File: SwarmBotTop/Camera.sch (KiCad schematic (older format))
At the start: 3 parts, among them J6 Conn_01x24_Female

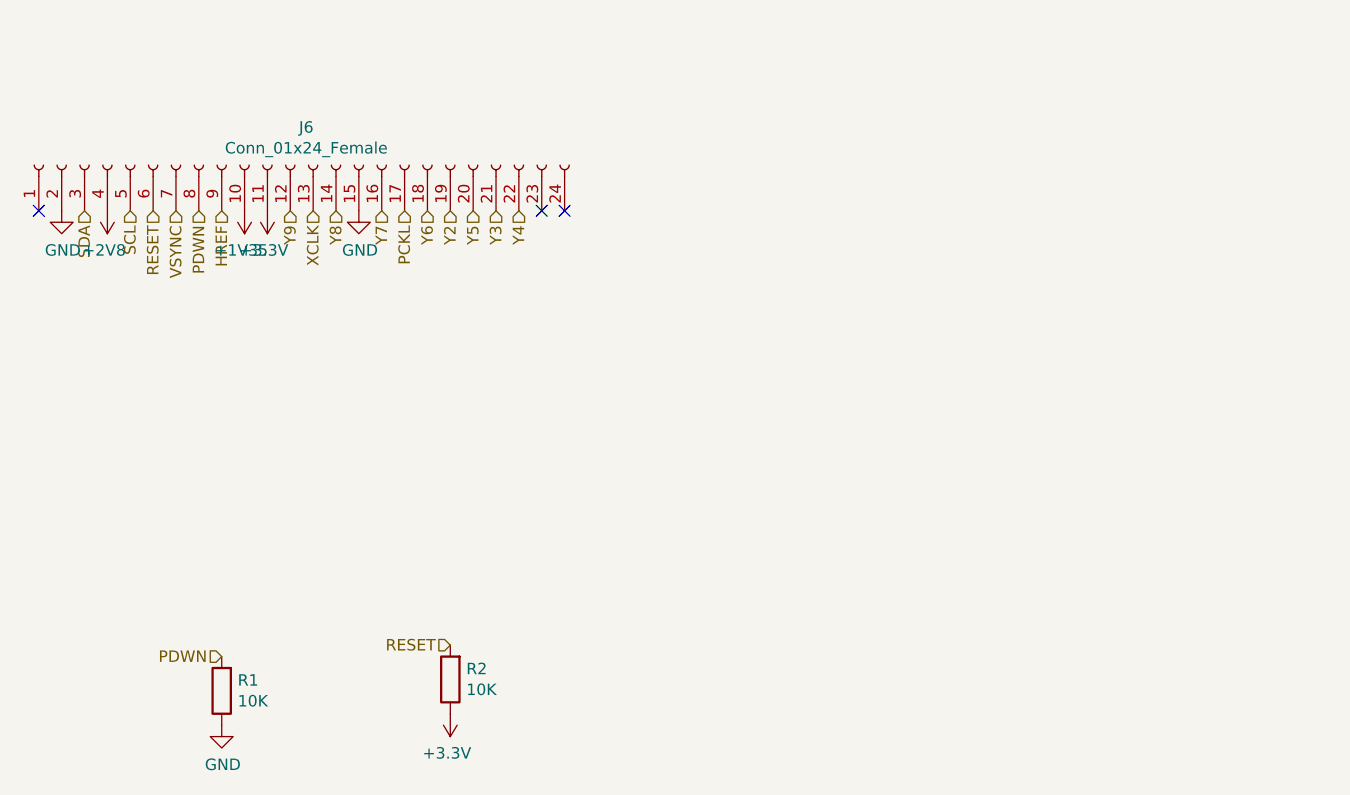
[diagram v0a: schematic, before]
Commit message: V1 ready to order
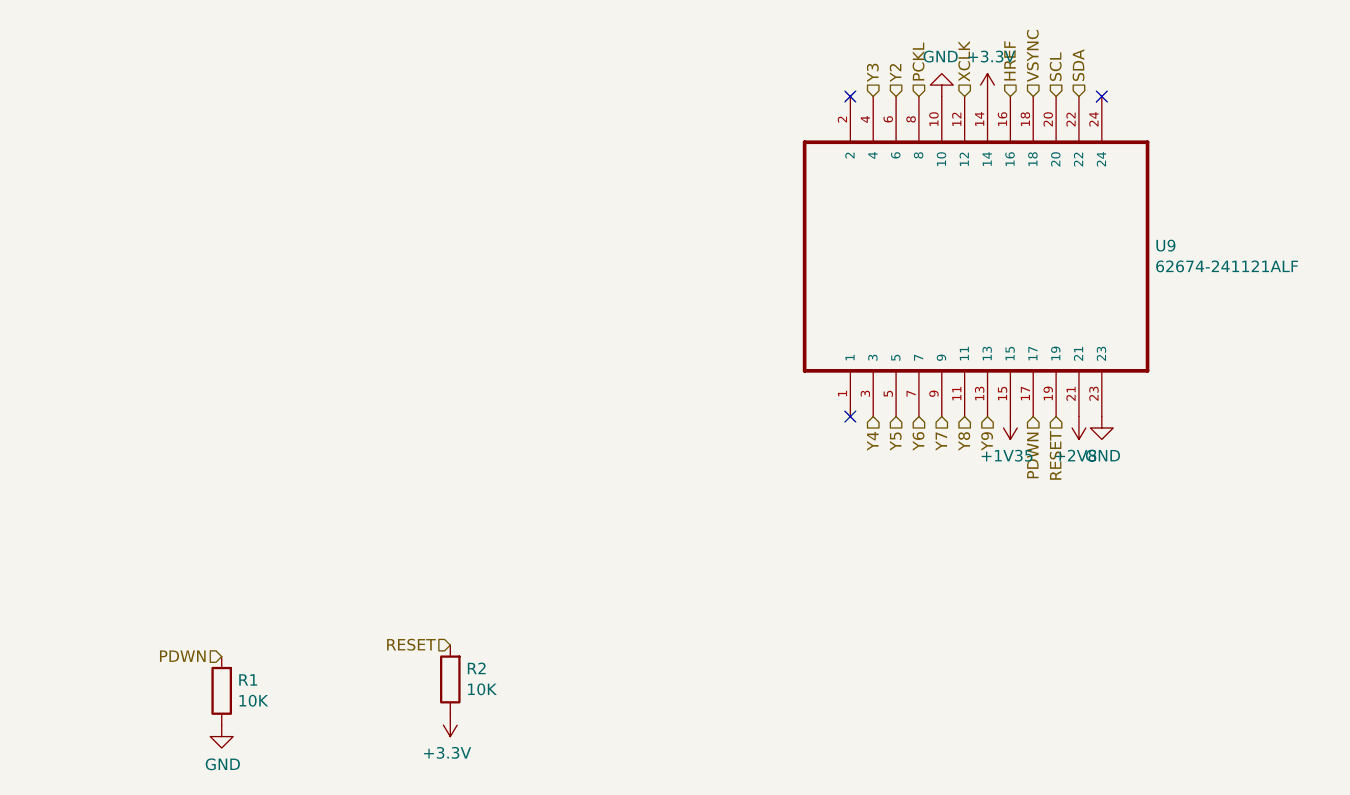
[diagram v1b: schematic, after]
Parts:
- removed J6: Conn_01x24_Female, Connector_FFC-FPC:Hirose_FH12-24S-0.5SH_1x24-1MP_P0.50mm_Horizontal, symbol Connector:Conn_01x24_Female
- added U9: 62674-241121ALF, ffc:FCI_62674-241121ALF, symbol 62674-241121ALF:62674-241121ALF
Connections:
- net +1V35: now also U9.15
- net +2V8: now also U9.21
- net +3V3: now also U9.14
- net GND: now also U9.10, U9.23
- net HREF: now also U9.16
- net PCKL: now also U9.8
- net PDWN: now also U9.17
- net RESET: now also U9.19
- net SCL: now also U9.20
- net SDA: now also U9.22
- net VSYNC: now also U9.18
- net XCLK: now also U9.12
- net Y2: now also U9.6
- net Y3: now also U9.4
- net Y4: now also U9.3
- net Y5: now also U9.5
- net Y6: now also U9.7
- net Y7: now also U9.9
- net Y8: now also U9.11
- net Y9: now also U9.13
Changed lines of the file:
@@
 $EndDescr
-$Comp
-L Connector:Conn_01x24_Female J6
-U 1 1 5DE89F78
-P 2550 1250
-F 0 "J6" V 2715 1180 50  0000 C CNN
-F 1 "Conn_01x24_Female" V 2624 1180 50  0000 C CNN
-F 2 "Connector_FFC-FPC:Hirose_FH12-24S-0.5SH_1x24-1MP_P0.50mm_Horizontal" H 2550 1250 50  0001 C CNN
-F 3 "~" H 2550 1250 50  0001 C CNN
-	1    2550 1250
-	0    -1   -1   0
-$EndComp
-NoConn ~ 3750 1450
-NoConn ~ 3650 1450
-NoConn ~ 1450 1450
-$Comp
-L power:GND #PWR0167
-U 1 1 5DE8C289
-P 2850 1450
-F 0 "#PWR0167" H 2850 1200 50  0001 C CNN
-F 1 "GND" H 2855 1277 50  0000 C CNN
-F 2 "" H 2850 1450 50  0001 C CNN
-F 3 "" H 2850 1450 50  0001 C CNN
-	1    2850 1450
-	1    0    0    -1
-$EndComp
-$Comp
-L power:GND #PWR0169
-U 1 1 5DE8C618
-P 1550 1450
-F 0 "#PWR0169" H 1550 1200 50  0001 C CNN
-F 1 "GND" H 1555 1277 50  0000 C CNN
-F 2 "" H 1550 1450 50  0001 C CNN
-F 3 "" H 1550 1450 50  0001 C CNN
-	1    1550 1450
-	1    0    0    -1
-$EndComp
-$Comp
-L power:+2V8 #PWR0170
-U 1 1 5DE8CB15
-P 1750 1450
-F 0 "#PWR0170" H 1750 1300 50  0001 C CNN
-F 1 "+2V8" H 1765 1623 50  0000 C CNN
-F 2 "" H 1750 1450 50  0001 C CNN
-F 3 "" H 1750 1450 50  0001 C CNN
-	1    1750 1450
-	-1   0    0    1
-$EndComp
-Text HLabel 1650 1450 3    50   Input ~ 0
-SDA
-Text HLabel 1850 1450 3    50   Input ~ 0
-SCL
-Text HLabel 1950 1450 3    50   Input ~ 0
-RESET
-Text HLabel 2050 1450 3    50   Input ~ 0
-VSYNC
-Text HLabel 2150 1450 3    50   Input ~ 0
-PDWN
-Text HLabel 2250 1450 3    50   Input ~ 0
-HREF
-$Comp
-L power:+1V35 #PWR0171
-U 1 1 5DE8D87F
-P 2350 1450
-F 0 "#PWR0171" H 2350 1300 50  0001 C CNN
-F 1 "+1V35" H 2365 1623 50  0000 C CNN
-F 2 "" H 2350 1450 50  0001 C CNN
-F 3 "" H 2350 1450 50  0001 C CNN
-	1    2350 1450
-	-1   0    0    1
-$EndComp
-$Comp
-L power:+3.3V #PWR0172
-U 1 1 5DE8DDE0
-P 2450 1450
-F 0 "#PWR0172" H 2450 1300 50  0001 C CNN
-F 1 "+3.3V" H 2465 1623 50  0000 C CNN
-F 2 "" H 2450 1450 50  0001 C CNN
-F 3 "" H 2450 1450 50  0001 C CNN
-	1    2450 1450
-	-1   0    0    1
-$EndComp
-Text HLabel 2550 1450 3    50   Input ~ 0
-Y9
-Text HLabel 2650 1450 3    50   Input ~ 0
-XCLK
-Text HLabel 2750 1450 3    50   Input ~ 0
-Y8
-Text HLabel 2950 1450 3    50   Input ~ 0
-Y7
-Text HLabel 3050 1450 3    50   Input ~ 0
-PCKL
-Text HLabel 3150 1450 3    50   Input ~ 0
-Y6
-Text HLabel 3350 1450 3    50   Input ~ 0
-Y5
-Text HLabel 3250 1450 3    50   Input ~ 0
-Y2
-Text HLabel 3450 1450 3    50   Input ~ 0
-Y3
-Text HLabel 3550 1450 3    50   Input ~ 0
-Y4
 $Comp
 L Device:R R1
@@
 	-1   0    0    1
 $EndComp
+NoConn ~ 5000 2350
+NoConn ~ 6100 950
+$Comp
+L power:GND #PWR0167
+U 1 1 5DFE7493
+P 5400 950
+F 0 "#PWR0167" H 5400 700 50  0001 C CNN
+F 1 "GND" H 5405 777 50  0000 C CNN
+F 2 "" H 5400 950 50  0001 C CNN
+F 3 "" H 5400 950 50  0001 C CNN
+	1    5400 950
+	-1   0    0    1
+$EndComp
+Text HLabel 5700 950  1    50   Input ~ 0
+HREF
+$Comp
+L power:+1V35 #PWR0169
+U 1 1 5DFE749A
+P 5700 2350
+F 0 "#PWR0169" H 5700 2200 50  0001 C CNN
+F 1 "+1V35" H 5715 2523 50  0000 C CNN
+F 2 "" H 5700 2350 50  0001 C CNN
+F 3 "" H 5700 2350 50  0001 C CNN
+	1    5700 2350
+	-1   0    0    1
+$EndComp
+$Comp
+L power:+3.3V #PWR0170
+U 1 1 5DFE74A0
+P 5600 950
+F 0 "#PWR0170" H 5600 800 50  0001 C CNN
+F 1 "+3.3V" H 5615 1123 50  0000 C CNN
+F 2 "" H 5600 950 50  0001 C CNN
+F 3 "" H 5600 950 50  0001 C CNN
+	1    5600 950
+	1    0    0    -1
+$EndComp
+Text HLabel 5600 2350 3    50   Input ~ 0
+Y9
+Text HLabel 5500 950  1    50   Input ~ 0
+XCLK
+Text HLabel 5500 2350 3    50   Input ~ 0
+Y8
+Text HLabel 5800 2350 3    50   Input ~ 0
+PDWN
+Text HLabel 5800 950  1    50   Input ~ 0
+VSYNC
+Text HLabel 5900 2350 3    50   Input ~ 0
+RESET
+Text HLabel 5900 950  1    50   Input ~ 0
+SCL
+$Comp
+L power:+2V8 #PWR0171
+U 1 1 5DFE74B9
+P 6000 2350
+F 0 "#PWR0171" H 6000 2200 50  0001 C CNN
+F 1 "+2V8" H 6015 2523 50  0000 C CNN
+F 2 "" H 6000 2350 50  0001 C CNN
+F 3 "" H 6000 2350 50  0001 C CNN
+	1    6000 2350
+	-1   0    0    1
+$EndComp
+Text HLabel 6000 950  1    50   Input ~ 0
+SDA
+$Comp
+L power:GND #PWR0172
+U 1 1 5DFE74C0
+P 6100 2350
+F 0 "#PWR0172" H 6100 2100 50  0001 C CNN
+F 1 "GND" H 6105 2177 50  0000 C CNN
+F 2 "" H 6100 2350 50  0001 C CNN
+F 3 "" H 6100 2350 50  0001 C CNN
+	1    6100 2350
+	1    0    0    -1
+$EndComp
+Text HLabel 5400 2350 3    50   Input ~ 0
+Y7
+Text HLabel 5300 950  1    50   Input ~ 0
+PCKL
+Text HLabel 5300 2350 3    50   Input ~ 0
+Y6
+Text HLabel 5200 950  1    50   Input ~ 0
+Y2
+Text HLabel 5200 2350 3    50   Input ~ 0
+Y5
+Text HLabel 5100 950  1    50   Input ~ 0
+Y3
+Text HLabel 5100 2350 3    50   Input ~ 0
+Y4
+$Comp
+L 62674-241121ALF:62674-241121ALF U9
+U 1 1 5DFB2785
+P 5400 1650
+F 0 "U9" V 5446 717 50  0000 R CNN
+F 1 "62674-241121ALF" V 5355 717 50  0000 R CNN
+F 2 "ffc:FCI_62674-241121ALF" H 5400 1650 50  0001 L BNN
+F 3 "62674-241121ALF" H 5400 1650 50  0001 L BNN
+F 4 "03M2162" H 5400 1650 50  0001 L BNN "Field4"
+F 5 "1830630" H 5400 1650 50  0001 L BNN "Field5"
+F 6 "FCI" H 5400 1650 50  0001 L BNN "Field6"
+F 7 "CONN-24POS" H 5400 1650 50  0001 L BNN "Field7"
+	1    5400 1650
+	0    -1   -1   0
+$EndComp
+NoConn ~ 5000 950
 $EndSCHEMATC
